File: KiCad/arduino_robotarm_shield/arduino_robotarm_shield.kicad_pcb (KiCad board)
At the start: 2 copper layers, 57.1 x 53.4 mm, 10 parts, among them J1 Screw_Terminal_01x02, J2 Conn_01x03, J3 Conn_01x03, J4 Conn_01x03, J5 Conn_01x03, J6 Conn_01x03, J7 Conn_01x03

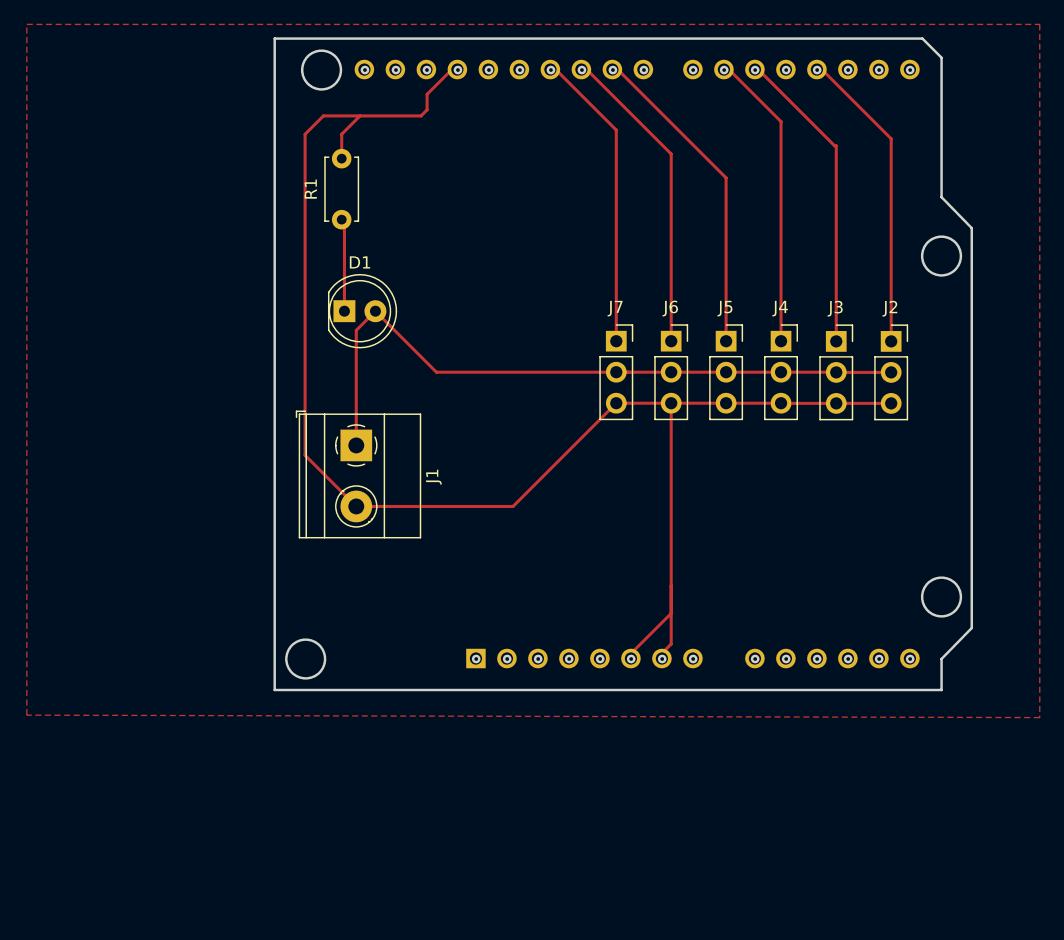
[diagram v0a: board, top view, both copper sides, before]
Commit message: Nov 23th
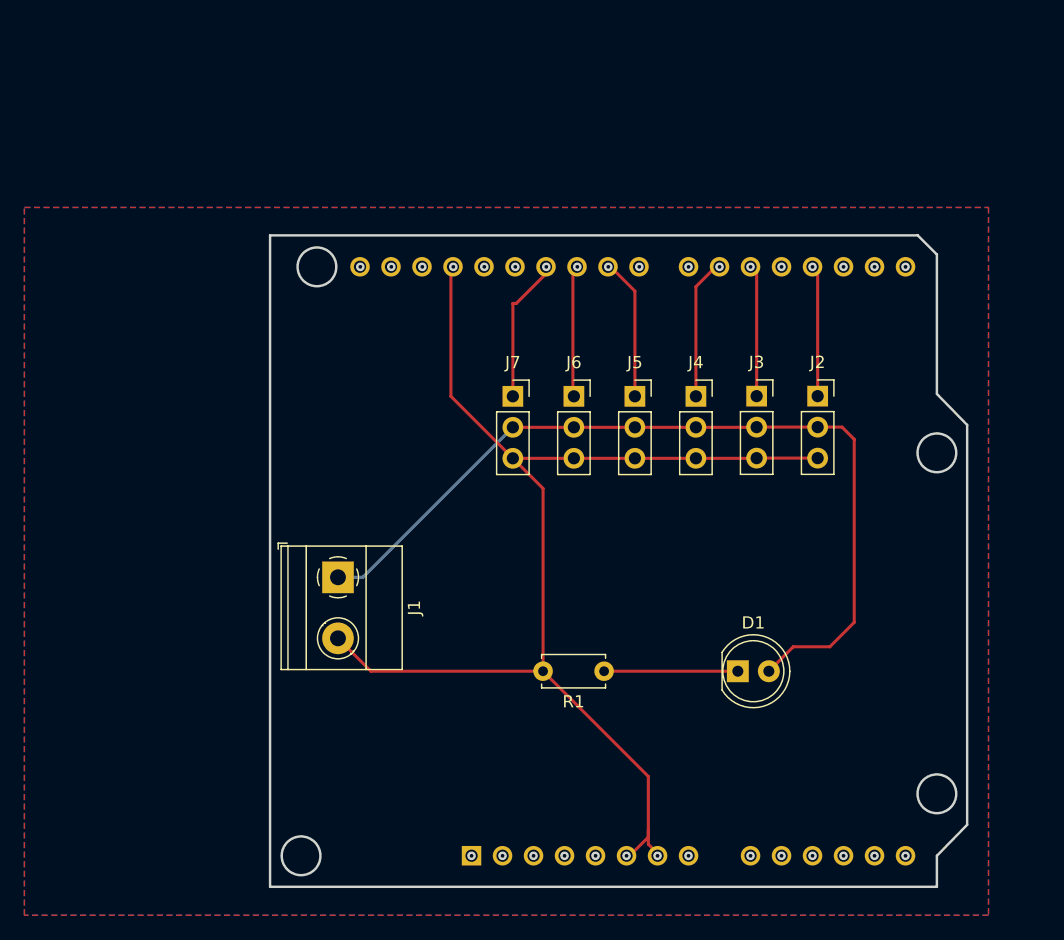
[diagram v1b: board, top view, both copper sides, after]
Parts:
- moved D1 43.7 mm to (165.5, 66.0)
- moved R1 42.8 mm to (154.5, 66.0), turned to 180 degrees
- moved A1 16.2 mm to (143.6, 81.1)
- moved J1 10.9 mm to (132.7, 58.3)
- moved J7 9.60 mm to (147.0, 43.5)
- moved J6 9.16 mm to (152.0, 43.5)
- moved J5 8.73 mm to (157.0, 43.5)
- moved J4 8.31 mm to (162.0, 43.5)
- moved J3 7.92 mm to (167.0, 43.5)
- moved J2 7.51 mm to (172.0, 43.5)
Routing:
- net GND: track 127.2 -> 100.3 mm
- net /S3: track 25.9 -> 11.1 mm
- net /S4: track 25.1 -> 10.6 mm
- net -5V: track 57.0 -> 71.5 mm
- net /S1: track 25.0 -> 10.6 mm
- net /S0: track 24.6 -> 10.5 mm
- net /S2: track 24.0 -> 11.2 mm
- net /S5: track 24.3 -> 12.1 mm
- net Net-(D1-K): track 7.59 -> 11.0 mm
- added copper zone on B.Cu, net GND
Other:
- outline, holes or cut-outs redrawn
